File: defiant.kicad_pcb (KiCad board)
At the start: 2 copper layers, 126.6 x 99.6 mm, 55 parts, among them J1 Conn_01x02_Pin, SW1 SW_Push, SW2 SW_Push, SW3 SW_DP3T, T0 SW_PUSH, T1 SW_PUSH, T2 SW_PUSH, T3 SW_PUSH, T4 SW_PUSH, U1 Seeed Studio XIAO BLE

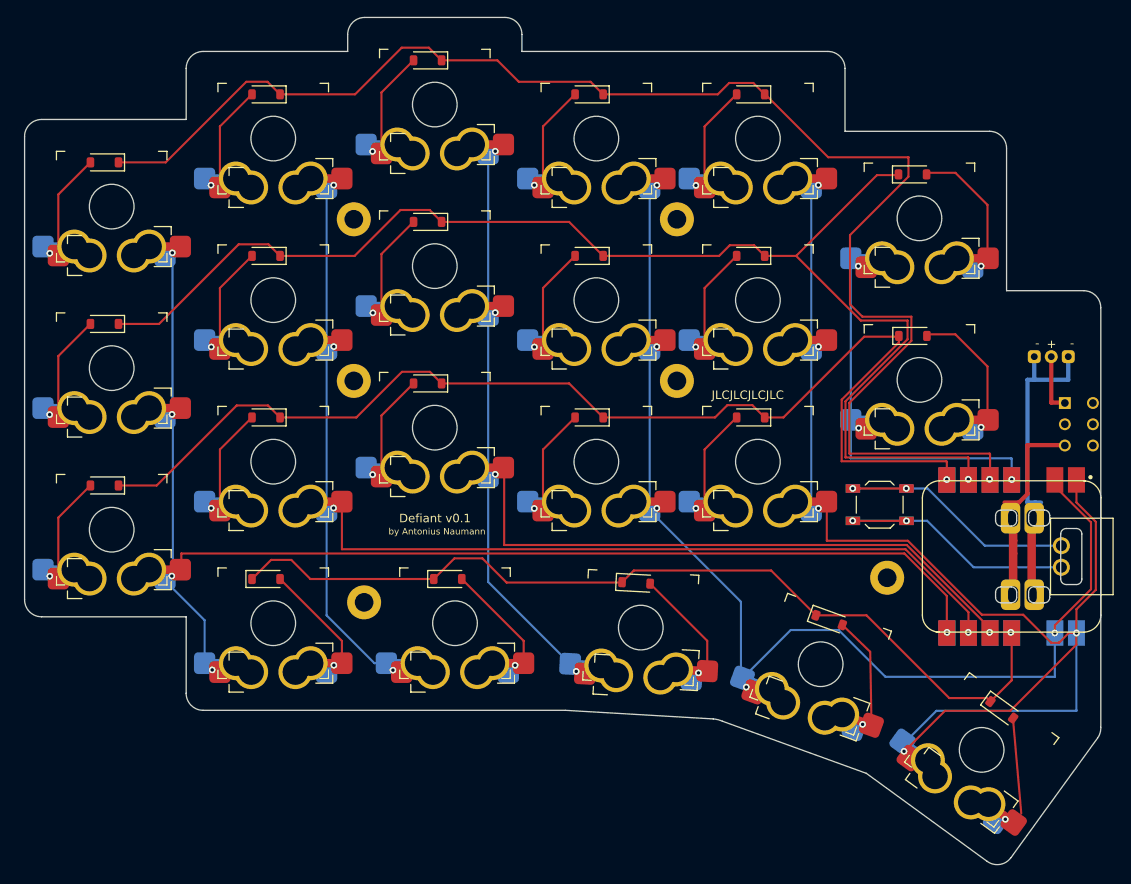
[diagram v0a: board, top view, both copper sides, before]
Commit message: Experimental: Tighten thumb key placing
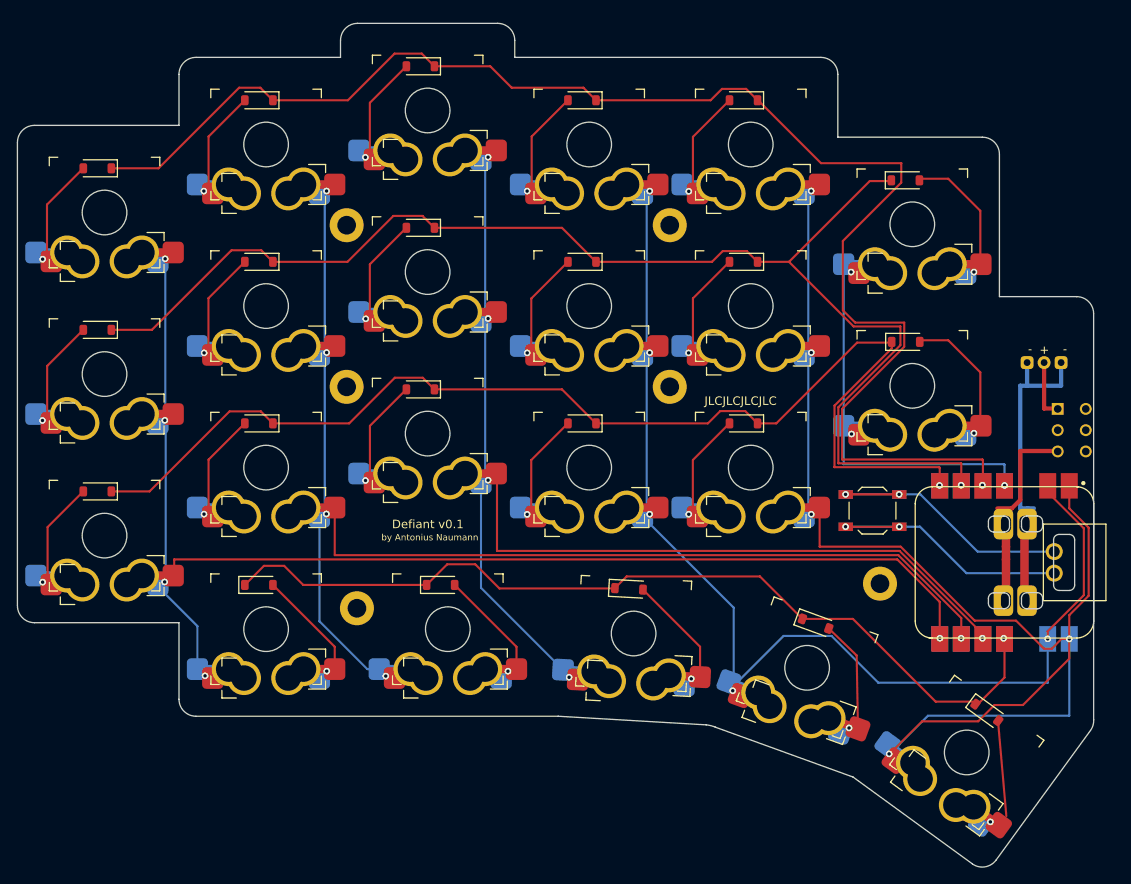
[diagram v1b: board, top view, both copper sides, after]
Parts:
- moved T4 1.78 mm to (190.6, 134.3)
- moved D20 1.78 mm to (192.9, 129.5)
- moved T3 1.65 mm to (171.8, 124.3)
- moved D16 1.65 mm to (172.8, 119.1)
- moved C0R1 1.09 mm to (89.2, 70.8)
- moved D14 1.09 mm to (145.3, 76.6)
- moved D8 1.09 mm to (128.7, 114.6)
- moved REF** 1.09 mm to (117.7, 91.3)
- moved C1R1 1.09 mm to (108.2, 62.8)
- moved C2R2 1.09 mm to (127.2, 77.8)
- moved C2R3 1.09 mm to (127.2, 96.8)
- moved D1 1.09 mm to (88.3, 65.6)
- moved D3 1.09 mm to (88.3, 103.6)
- moved J1 1.09 mm to (199.7, 88.4)
- moved D9 1.09 mm to (126.3, 53.6)
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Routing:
- net row3: track 107.0 -> 105.5 mm
- net col4: track 155.7 -> 156.8 mm
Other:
- board size 126.6 x 99.6 mm -> 126.6 x 99.2 mm
